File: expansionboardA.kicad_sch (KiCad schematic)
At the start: 66 parts, among them J1 DEBUG, J2 USB_A_Stacked, J3 HDMI_A, J4 FAN, J5 Conn_02x06_Odd_Even, J6 Conn_02x06_Odd_Even, J7 DEBUG, P1 USB_C_Plug, U1 MAX3420EECJ, U2 GPIO_U2, U4 GPIO_U4, U5 MCP3008T-I/SL, U6 CS4344-CZZR, U7 MAX3421EEHJ+T, Y1 Crystal, Y2 Crystal

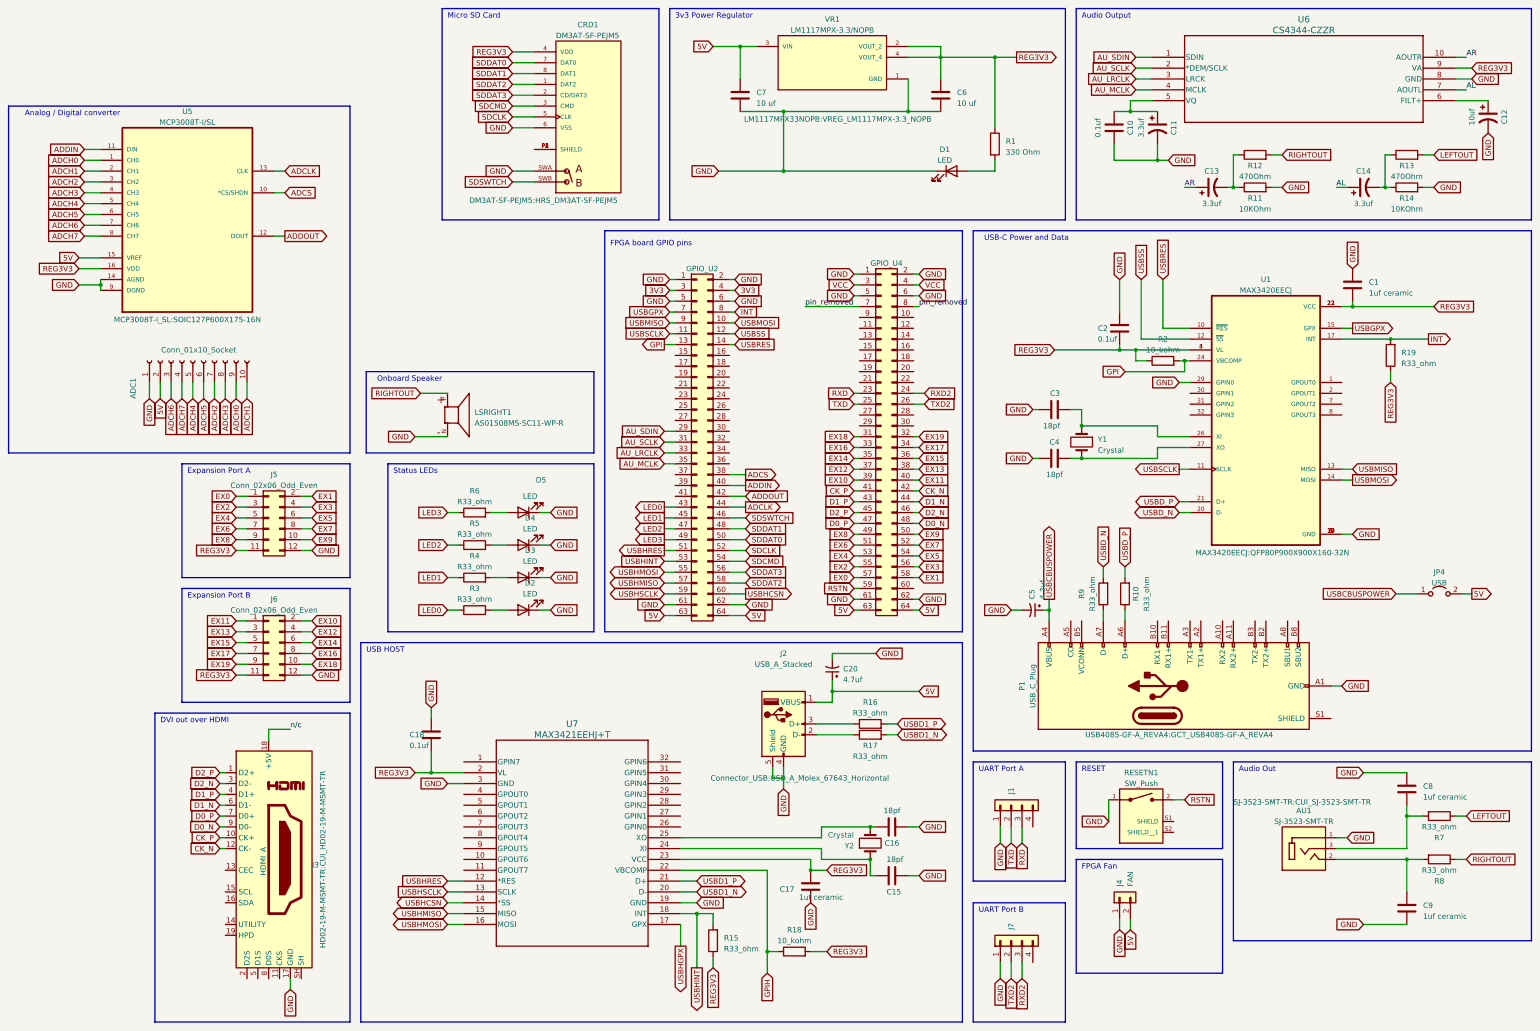
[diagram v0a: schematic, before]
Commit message: mods
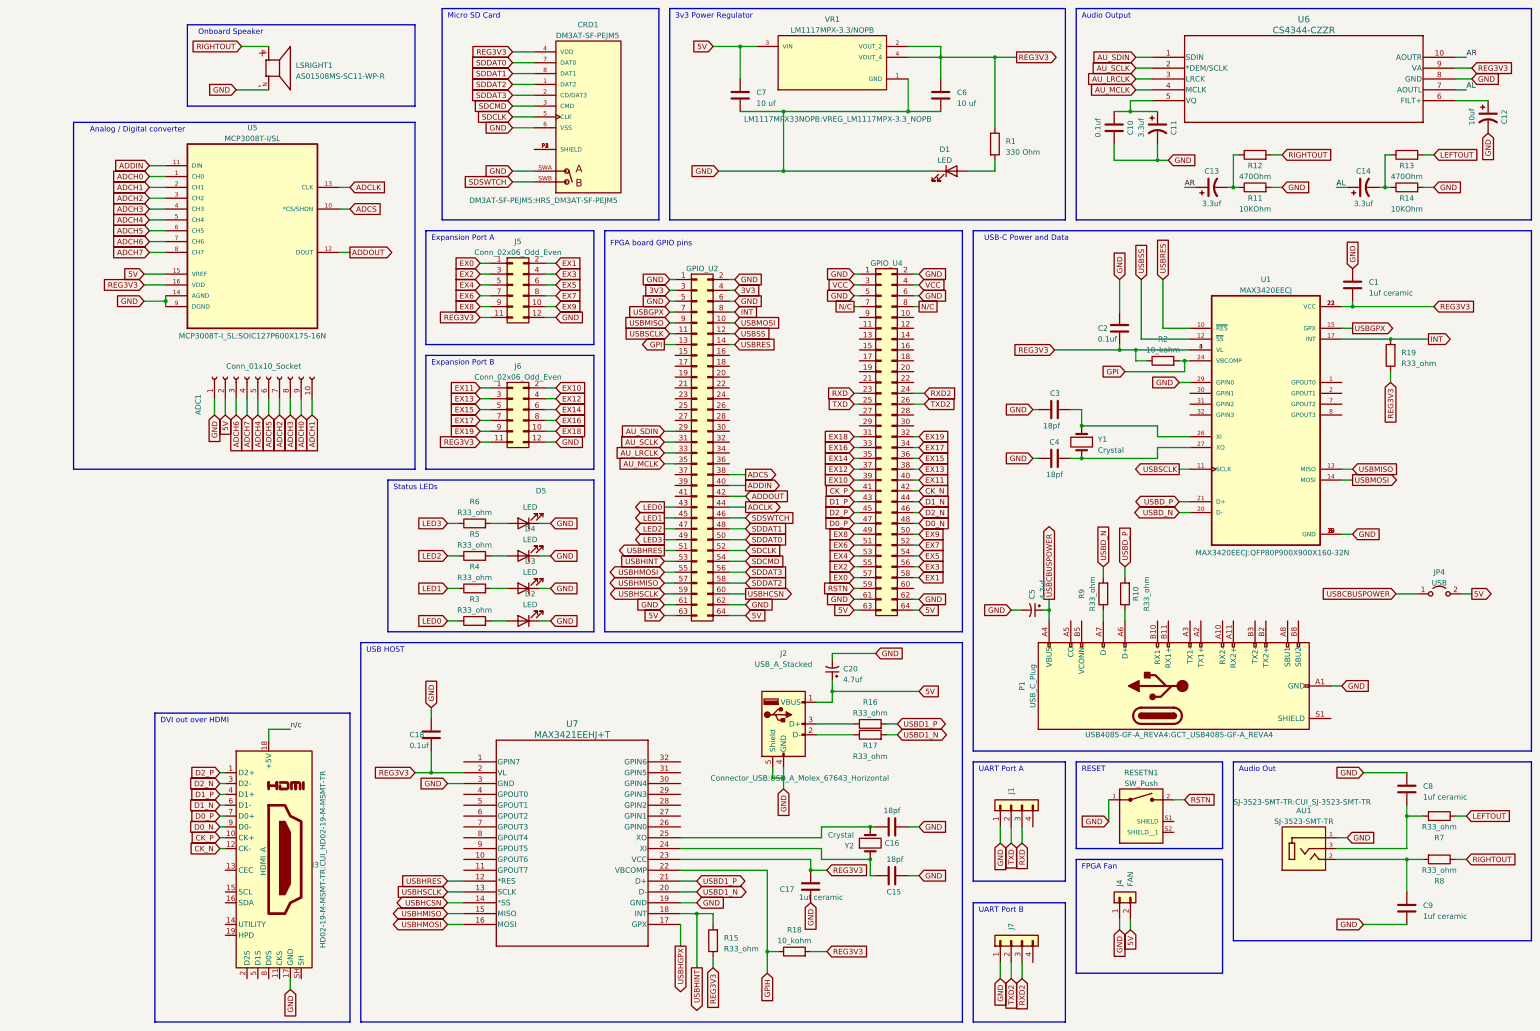
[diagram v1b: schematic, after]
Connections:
- net pin_removed renamed N/C
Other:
- moved on the sheet: ADC1, D2, D3, D4, D5, J5, J6, LSRIGHT1, R3, R4, R5, R6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

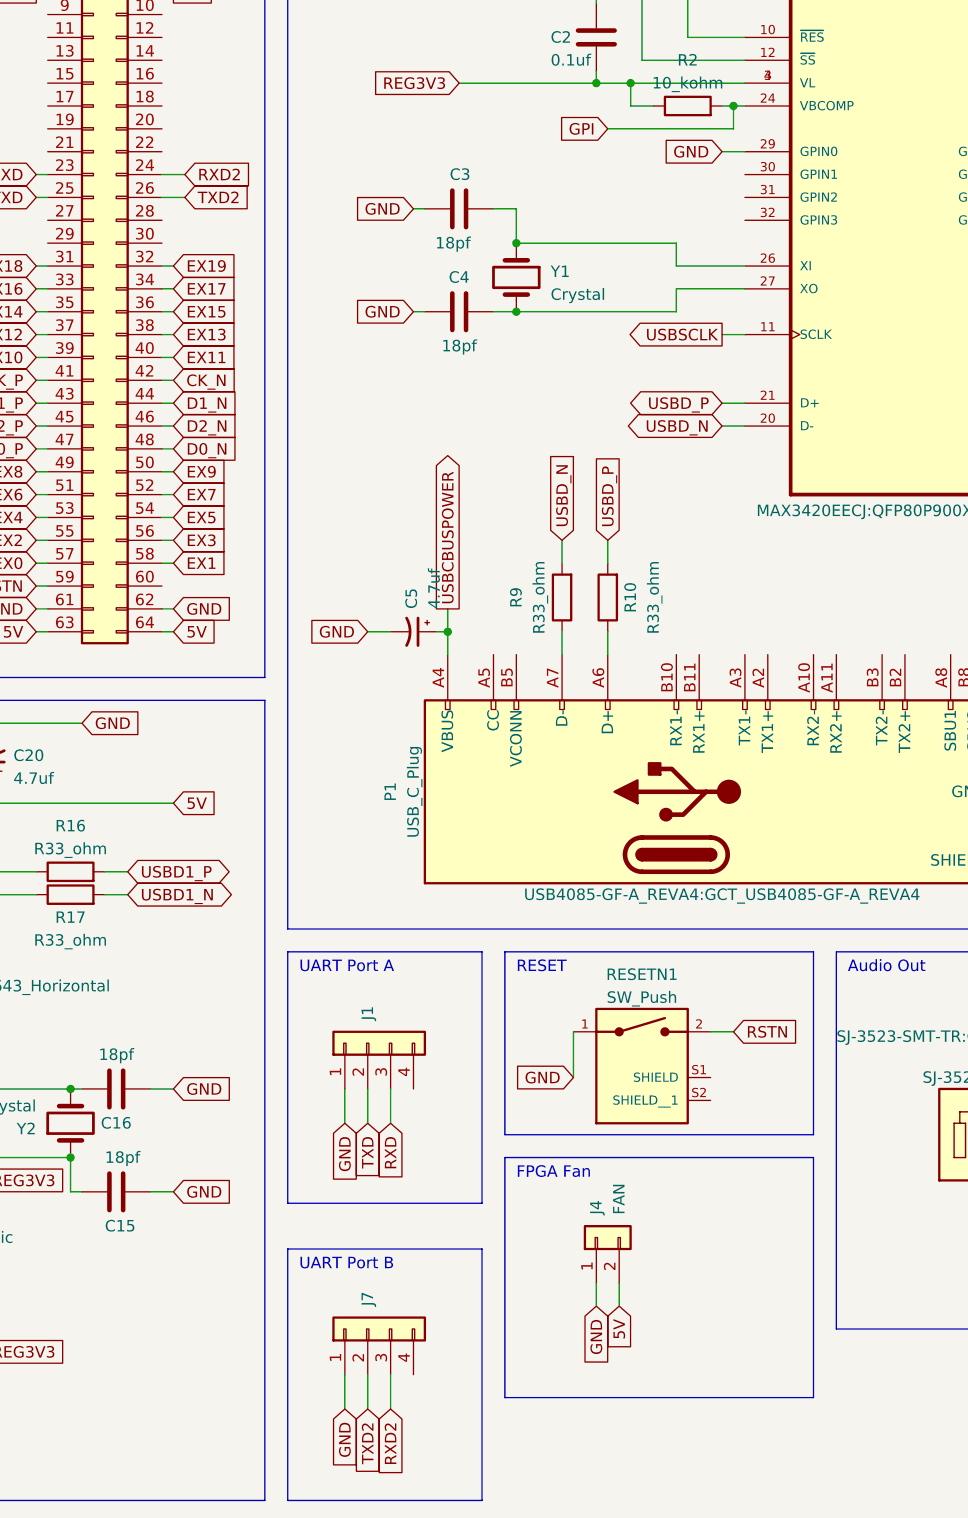
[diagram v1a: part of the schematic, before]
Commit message: Updated board
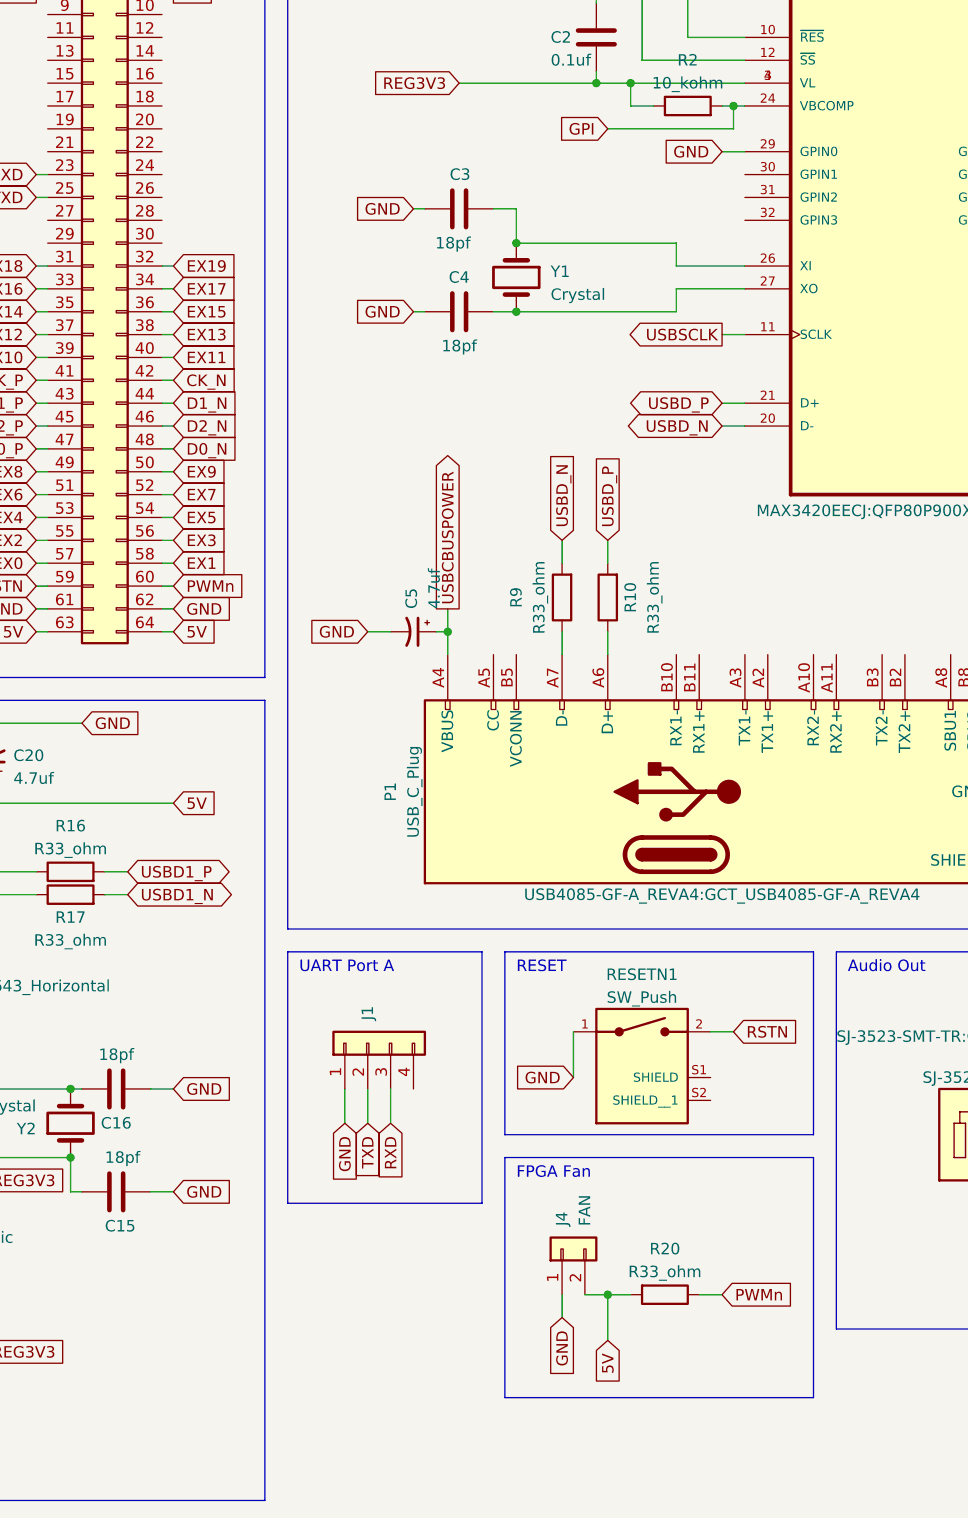
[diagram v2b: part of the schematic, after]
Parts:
- removed J7: DEBUG, Connector_PinSocket_2.54mm:PinSocket_1x04_P2.54mm_Vertical, symbol Connector_Generic:Conn_01x04
- added R20: R33_ohm, Resistor_SMD:R_0603_1608Metric_Pad0.98x0.95mm_HandSolder, symbol Device:R
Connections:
- net 5V: now also R20.2
- net PWMn: now reaches U4.60 (Pin_60)
- net PWMn: now also R20.1
- net RXD2: no longer names the net of U4.24 (Pin_24)
- net TXD2: no longer names the net of U4.26 (Pin_26)
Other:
- note removed: "UART Port B"
- moved on the sheet: J4
